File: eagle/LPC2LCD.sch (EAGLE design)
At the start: 7 parts, among them IC1 LC4032V-75TN44C

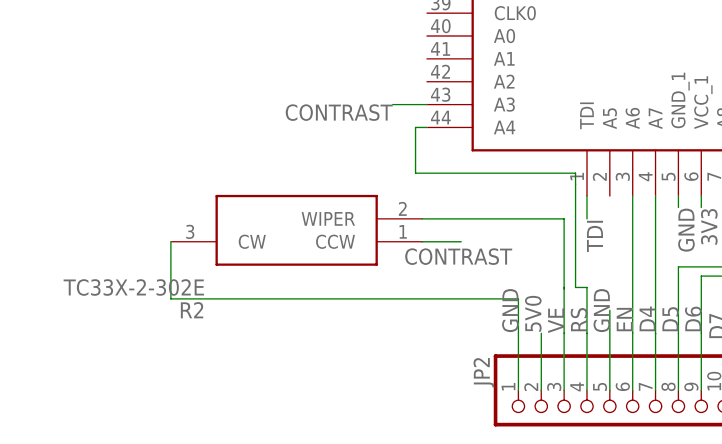
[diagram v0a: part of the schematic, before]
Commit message: Add files via upload
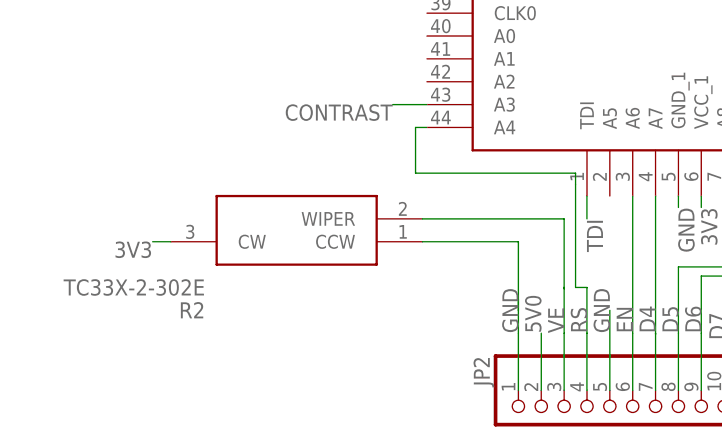
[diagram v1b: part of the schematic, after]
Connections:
- net 3V3: now also R2.CW
- net CONTRAST: no longer R2.CCW
- net GND: now also R2.CCW; no longer R2.CW
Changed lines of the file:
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@@
 <label x="55.88" y="73.66" size="1.778" layer="95" rot="R90"/>
+</segment>
+<segment>
+<pinref part="R2" gate="G$1" pin="CW"/>
+<wire x1="9.652" y1="25.4" x2="7.62" y2="25.4" width="0.1524" layer="91"/>
+<label x="7.62" y="25.4" size="1.778" layer="95" rot="R180"/>
 </segment>
 </net>
@@
 <wire x1="48.26" y1="8.89" x2="48.26" y2="15.24" width="0.1524" layer="91"/>
 <label x="48.26" y="15.24" size="1.778" layer="95" rot="R90"/>
-<pinref part="R2" gate="G$1" pin="CW"/>
-<wire x1="9.652" y1="25.4" x2="9.652" y2="19.05" width="0.1524" layer="91"/>
-<wire x1="9.652" y1="19.05" x2="48.26" y2="19.05" width="0.1524" layer="91"/>
-<wire x1="48.26" y1="19.05" x2="48.26" y2="15.24" width="0.1524" layer="91"/>
+<wire x1="48.26" y1="19.05" x2="48.26" y2="17.78" width="0.1524" layer="91"/>
 <pinref part="JP2" gate="G$1" pin="1"/>
+<pinref part="R2" gate="G$1" pin="CCW"/>
+<wire x1="48.26" y1="17.78" x2="48.26" y2="15.24" width="0.1524" layer="91"/>
+<wire x1="37.592" y1="25.4" x2="48.26" y2="25.4" width="0.1524" layer="91"/>
+<wire x1="48.26" y1="25.4" x2="48.26" y2="17.78" width="0.1524" layer="91"/>
 </segment>
 <segment>
@@
 <label x="34.29" y="40.64" size="1.778" layer="95" rot="R180"/>
 </segment>
-<segment>
-<pinref part="R2" gate="G$1" pin="CCW"/>
-<wire x1="37.592" y1="25.4" x2="41.91" y2="25.4" width="0.1524" layer="91"/>
-<label x="35.56" y="22.86" size="1.778" layer="95"/>
-</segment>
-</net>
+</net>
